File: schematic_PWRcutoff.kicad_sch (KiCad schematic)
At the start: 35 parts, among them J1 Conn_01x04, J10 Conn_01x02, J11 Conn_01x02, J2 Conn_01x04, J3 Conn_01x02, J4 Conn_01x08, J5 Conn_01x08, J6 Conn_01x02, J7 Conn_01x02, J8 Conn_01x02, J9 Conn_01x02, Q1 Q_PMOS_GSD, Q7 Q_PMOS_GSD, SW1 SW_SPST, SW3 SW_SPST, U1 MCP2562-H-SN

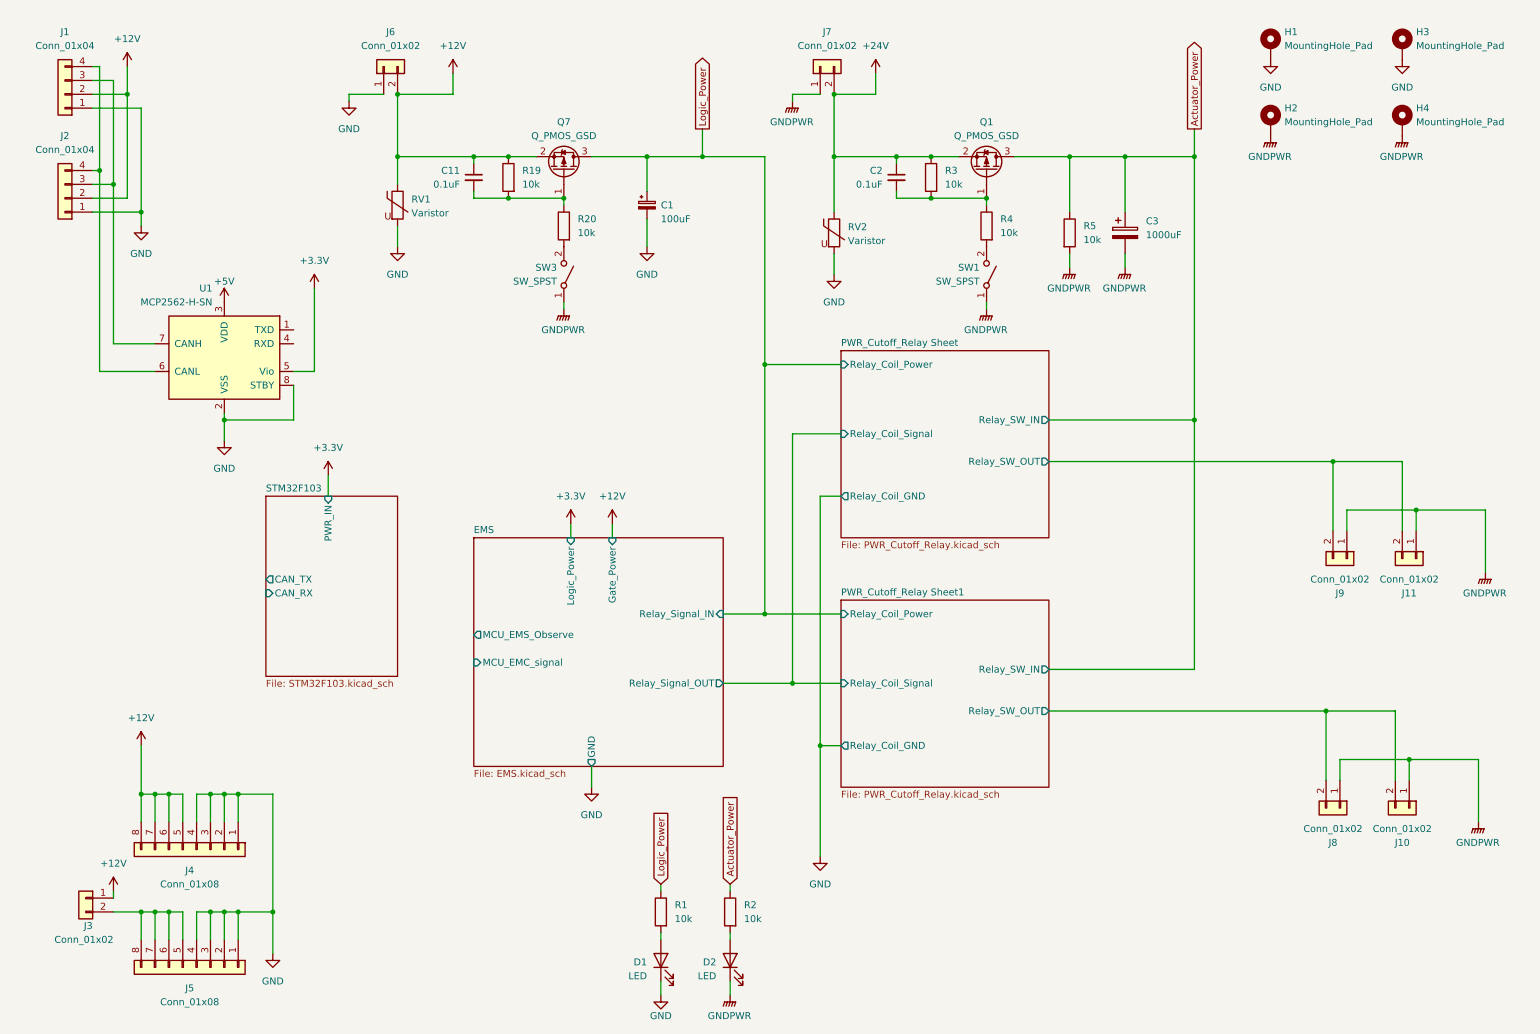
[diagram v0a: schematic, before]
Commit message: precompreate design
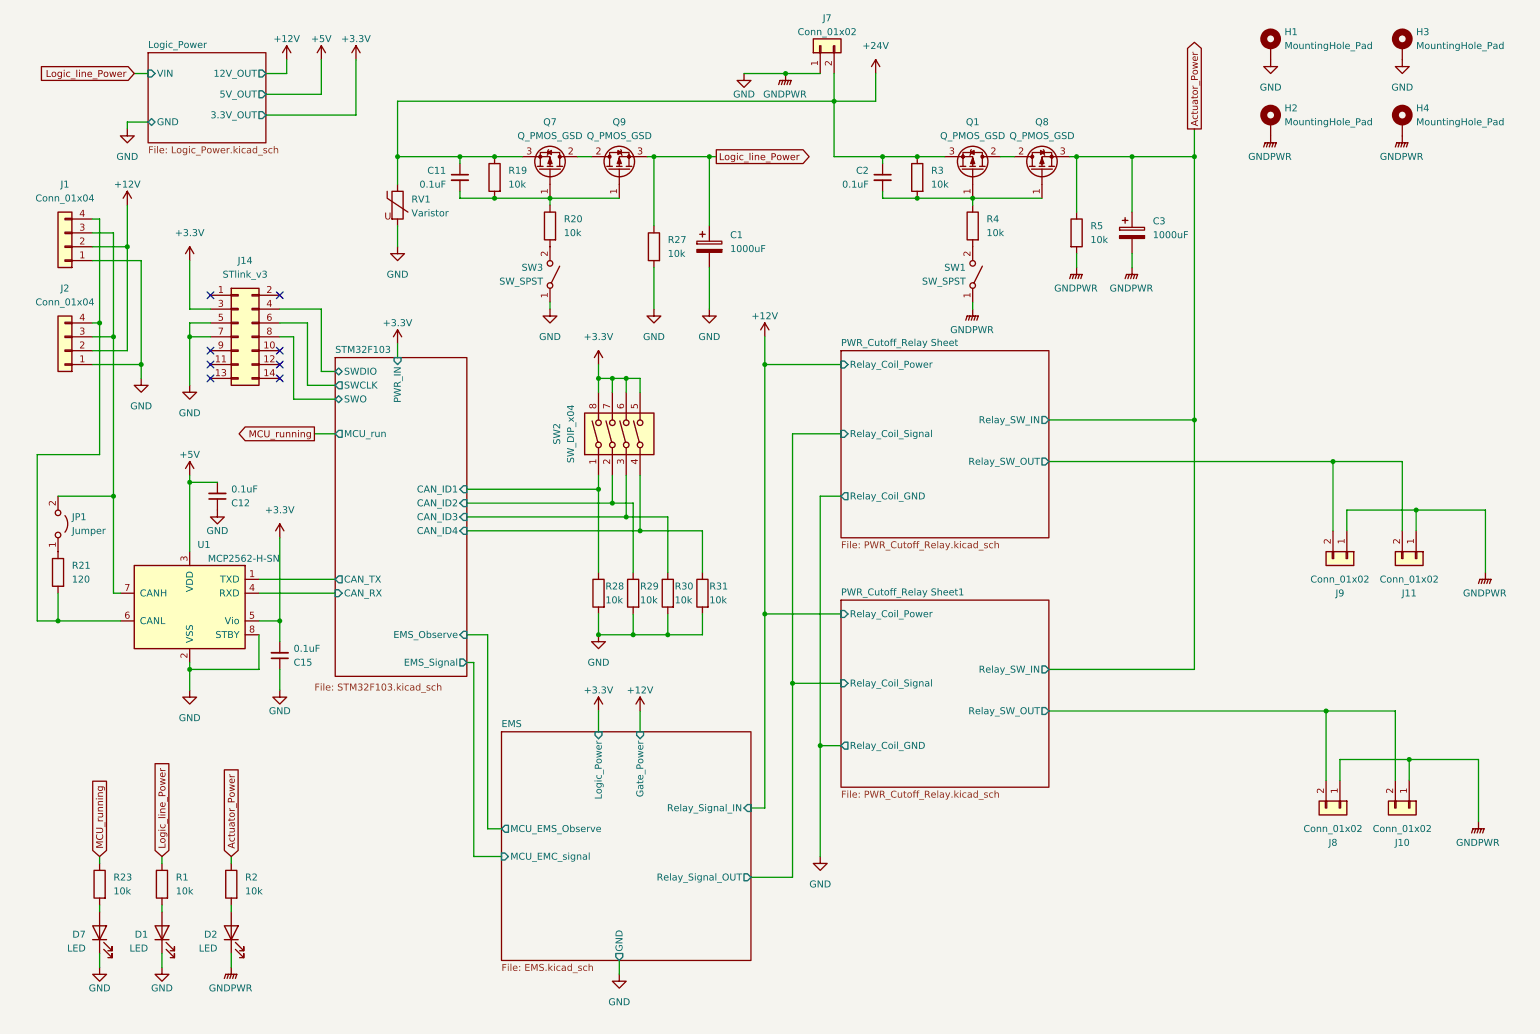
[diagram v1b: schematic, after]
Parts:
- removed C1: 100uF, Capacitor_THT:CP_Radial_D8.0mm_P5.00mm, symbol Device:C_Polarized_Small
- removed J3: Conn_01x02, Connector_PinHeader_2.54mm:PinHeader_1x02_P2.54mm_Vertical, symbol Connector_Generic:Conn_01x02
- removed J4, J5: Conn_01x08, Connector_PinHeader_2.54mm:PinHeader_1x08_P2.54mm_Vertical, symbol Connector_Generic:Conn_01x08
- removed J6: Conn_01x02, Connector_AMASS:AMASS_XT60-M_1x02_P7.20mm_Vertical, symbol Connector_Generic:Conn_01x02
- removed Q1: Q_PMOS_GSD, Package_TO_SOT_THT:TO-3P-3_Vertical, symbol Device:Q_PMOS_GSD
- removed RV2: Varistor, Varistor:RV_Disc_D12mm_W4.5mm_P7.5mm, symbol Device:Varistor
- added C1: 1000uF, Capacitor_THT:CP_Radial_D16.0mm_P7.50mm, symbol Device:C_Polarized
- added C12, C15: 0.1uF, Capacitor_SMD:C_0603_1608Metric_Pad1.08x0.95mm_HandSolder, symbol Device:C_Small
- added D7: LED, LED_SMD:LED_0603_1608Metric_Pad1.05x0.95mm_HandSolder, symbol Device:LED
- added J14: STlink_v3, RDC_general:JTAG_box_connector, symbol Connector_Generic:Conn_02x07_Odd_Even
- added JP1: Jumper, Connector_PinHeader_2.54mm:PinHeader_1x02_P2.54mm_Vertical, symbol Jumper:Jumper_2_Open
- added Q1, Q8, Q9: Q_PMOS_GSD, Package_TO_SOT_SMD:TO-252-2, symbol Device:Q_PMOS_GDS
- added R21: 120, Resistor_SMD:R_0603_1608Metric_Pad0.98x0.95mm_HandSolder, symbol Device:R
- added R23, R27, R28, R29, R30, R31: 10k, Resistor_SMD:R_0603_1608Metric_Pad0.98x0.95mm_HandSolder, symbol Device:R
- added SW2: SW_DIP_x04, Button_Switch_SMD:SW_DIP_SPSTx04_Slide_Copal_CHS-04B_W7.62mm_P1.27mm, symbol Switch:SW_DIP_x04
- C3: footprint Capacitor_THT:CP_Radial_D18.0mm_P7.50mm -> Capacitor_THT:CP_Radial_D16.0mm_P7.50mm
- Q7: footprint Package_TO_SOT_THT:TO-3P-3_Vertical -> Package_TO_SOT_SMD:TO-252-2; symbol Device:Q_PMOS_GSD -> Device:Q_PMOS_GDS
- RV1: footprint Varistor:RV_Disc_D12mm_W4.5mm_P7.5mm -> Varistor:RV_Disc_D9mm_W4.5mm_P5mm
- SW1, SW3: footprint (none) -> RDC_general:Toggle_switch
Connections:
- net GNDPWR is gone; now on net GND: C3.2, D2.1 (K), H2.1, H4.1, J10.1 (Pin_1), J11.1 (Pin_1), J7.1 (Pin_1), J8.1 (Pin_1), J9.1 (Pin_1), R5.2, SW1.1 (A), SW3.1 (A)
- net +12V: no longer C11.1, Q7.2 (S), R19.1, RV1.1
- net +24V: now also C11.1, Q7.3 (S), R19.1, RV1.1, Q1.3 (S)
- net +3.3V: now also C15.2, J14.3 (Pin_3), SW2.5, SW2.6, SW2.7, SW2.8
- net +5V: now also C12.2
- net Actuator_Power: now also Q8.3 (S)
- net GND: now also C1.2, C12.1, C15.1, D7.1 (K), J14.5 (Pin_5), J14.7 (Pin_7), R27.2, R28.2, R29.2, R30.2, R31.2
- net STM32F103/CAN_RX: now also U1.4 (RXD)
- net STM32F103/CAN_TX: now also U1.1 (TXD)
- net at J1.4 (Pin_4), J2.4 (Pin_4), U1.6 (CANL): now also R21.2
- net at J1.3 (Pin_3), J2.3 (Pin_3), U1.7 (CANH): now also JP1.2 (B)
- net at C11.2, Q7.1 (G), R19.2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: now also Q9.1 (G)
- net at C2.2, R3.2, R4.1: now also Q1.1 (G), Q8.1 (G)
- net Logic_Power renamed Logic_line_Power
- net Logic_line_Power: now also C1.1, Q9.3 (S), R27.1; no longer Q7.3 (D)
- new net: Q7.2 (D), Q9.2 (D)
- new net: D7.2 (A), R23.2
- new net: Q1.2 (D), Q8.2 (D)
- new net: JP1.1 (A), R21.1
- new net MCU_running: R23.1
- new net STM32F103/CAN_ID1: R28.1, SW2.1
- new net STM32F103/CAN_ID2: R29.1, SW2.2
- new net STM32F103/CAN_ID3: R30.1, SW2.3
- new net STM32F103/CAN_ID4: R31.1, SW2.4
- new net STM32F103/SWCLK: J14.6 (Pin_6)
- new net STM32F103/SWDIO: J14.4 (Pin_4)
- new net STM32F103/SWO: J14.8 (Pin_8)
- no-connect marks 0 -> 8
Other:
- added sheet Logic_Power (Logic_Power.kicad_sch)
- sheet STM32F103 ports: added CAN_ID1, CAN_ID2, CAN_ID3, CAN_ID4, EMS_Observe, EMS_Signal, MCU_run, SWCLK, SWDIO, SWO; removed none
- moved on the sheet: C11, C2, C3, D1, D2, J1, J2, J7, Q7, R1, R19, R2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
